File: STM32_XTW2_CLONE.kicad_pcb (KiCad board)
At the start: 2 copper layers, 81.3 x 28 mm, 27 parts, among them J1 USB A MALE, J2 ST-LINK, SW1 RST, U1 STM32F103C8Tx, U2 AMS1117-3.3, Y1 8Mhz

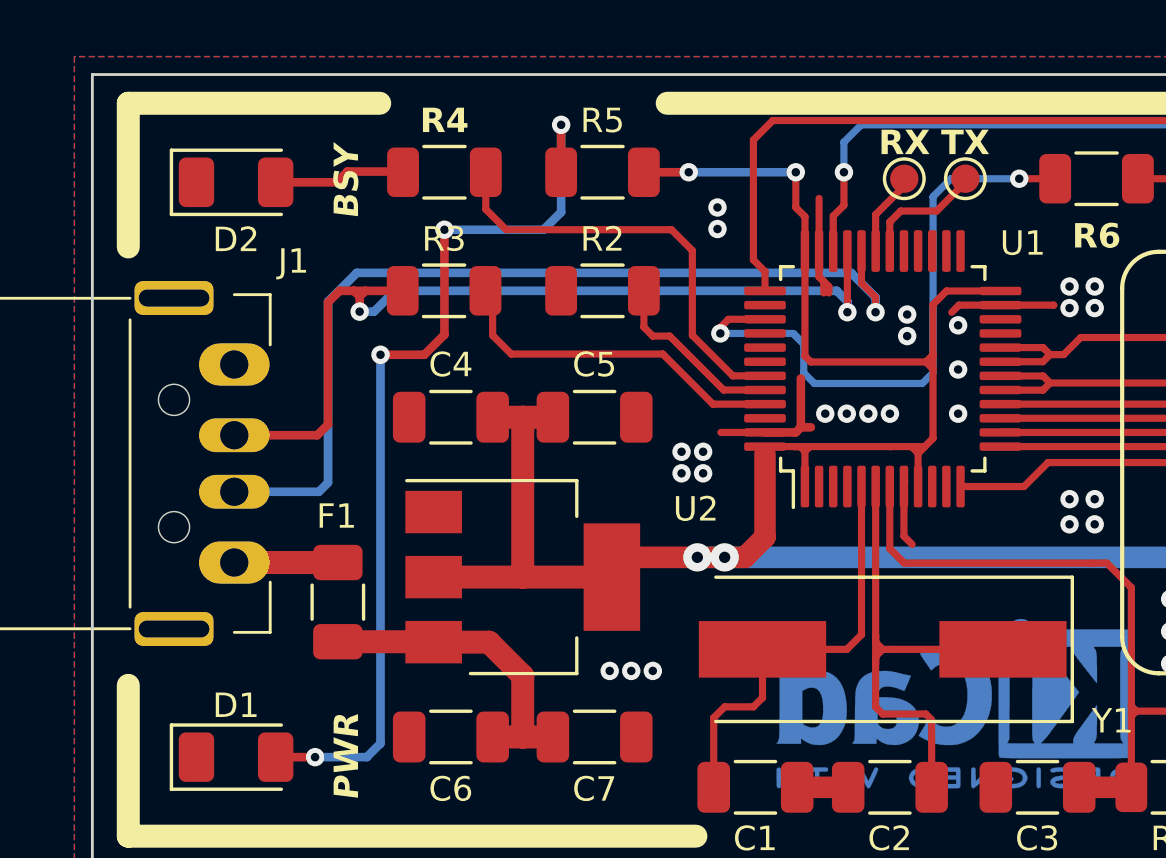
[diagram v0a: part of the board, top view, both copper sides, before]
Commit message: 25/03/23/C
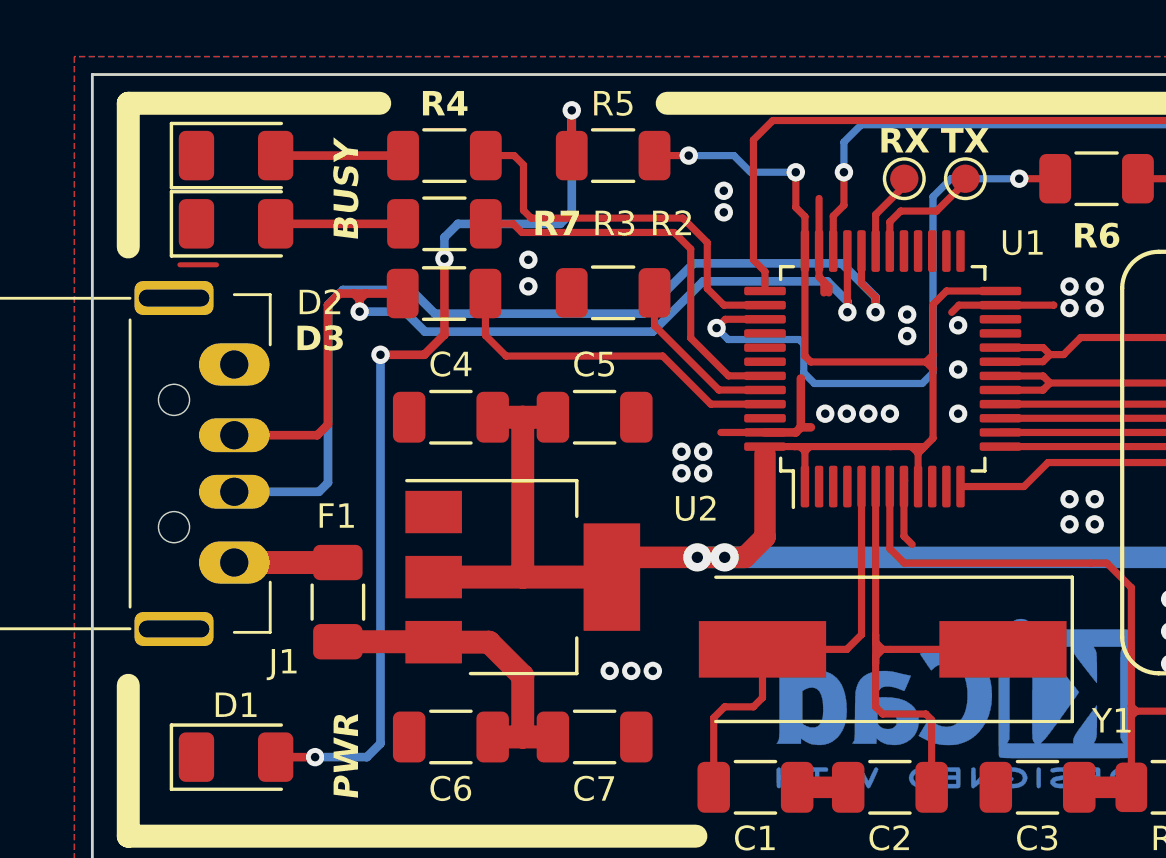
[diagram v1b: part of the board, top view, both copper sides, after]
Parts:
- added D3: LED, LED_SMD:LED_1206_3216Metric, F.Cu at (112.9, 103.4)
- added R7: 1K, Resistor_SMD:R_1206_3216Metric, F.Cu at (120.2, 103.4)
- moved D2 0.94 mm to (112.9, 101.0)
- moved R5 0.70 mm to (126.2, 101.0)
- moved R4 0.59 mm to (120.2, 101.0)
- moved R2 0.38 mm to (126.2, 105.8)
- moved R3 0.10 mm to (120.2, 105.8)
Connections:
- R4 pad 2: Net-(U1-PB7) -> Net-(U1-PA15)
- U1 pad 38: unconnected-(U1-PA15-Pad38) -> Net-(U1-PA15)
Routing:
- net Net-(U1-PA15): track 0.00 -> 14.0 mm
- net Net-(D3-A): track 0.00 -> 4.50 mm
- net Net-(D1-A): track 32.4 -> 33.7 mm
- net GND: track 29.0 -> 30.3 mm, vias 71 -> 73
- net Net-(U1-PB7): track 15.1 -> 13.9 mm
- net USB_N: track 32.9 -> 33.8 mm
- net Net-(U1-BOOT0): track 6.87 -> 6.01 mm
- net USB_P: track 32.0 -> 32.7 mm
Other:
- board text added: "BUSY"
- board text removed: "BSY"
